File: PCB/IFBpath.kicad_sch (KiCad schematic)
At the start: 51 parts, among them J401 NC3FAH2, J402 Conn_01x03, J403 Conn_01x03, J404 Conn_01x03, J405 Conn_01x03, J406 NRJ6HF, J407 NRJ6HF, U401 THAT2162, U402 OPA1678, U403 OPA1622

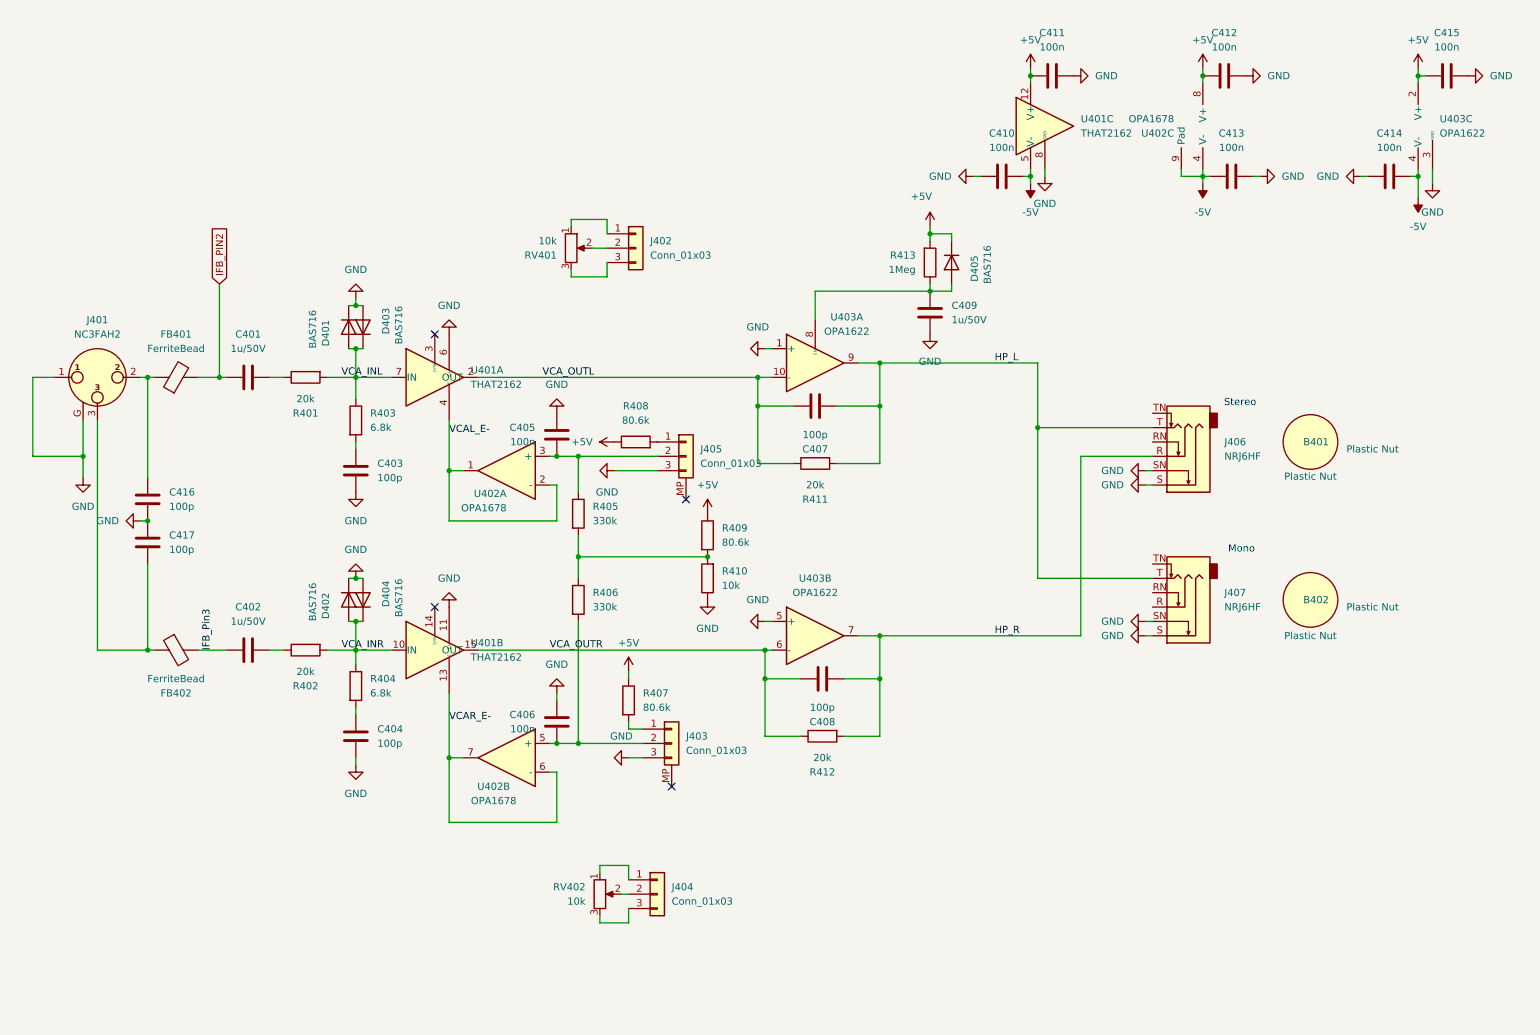
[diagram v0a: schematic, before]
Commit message: Tidying up
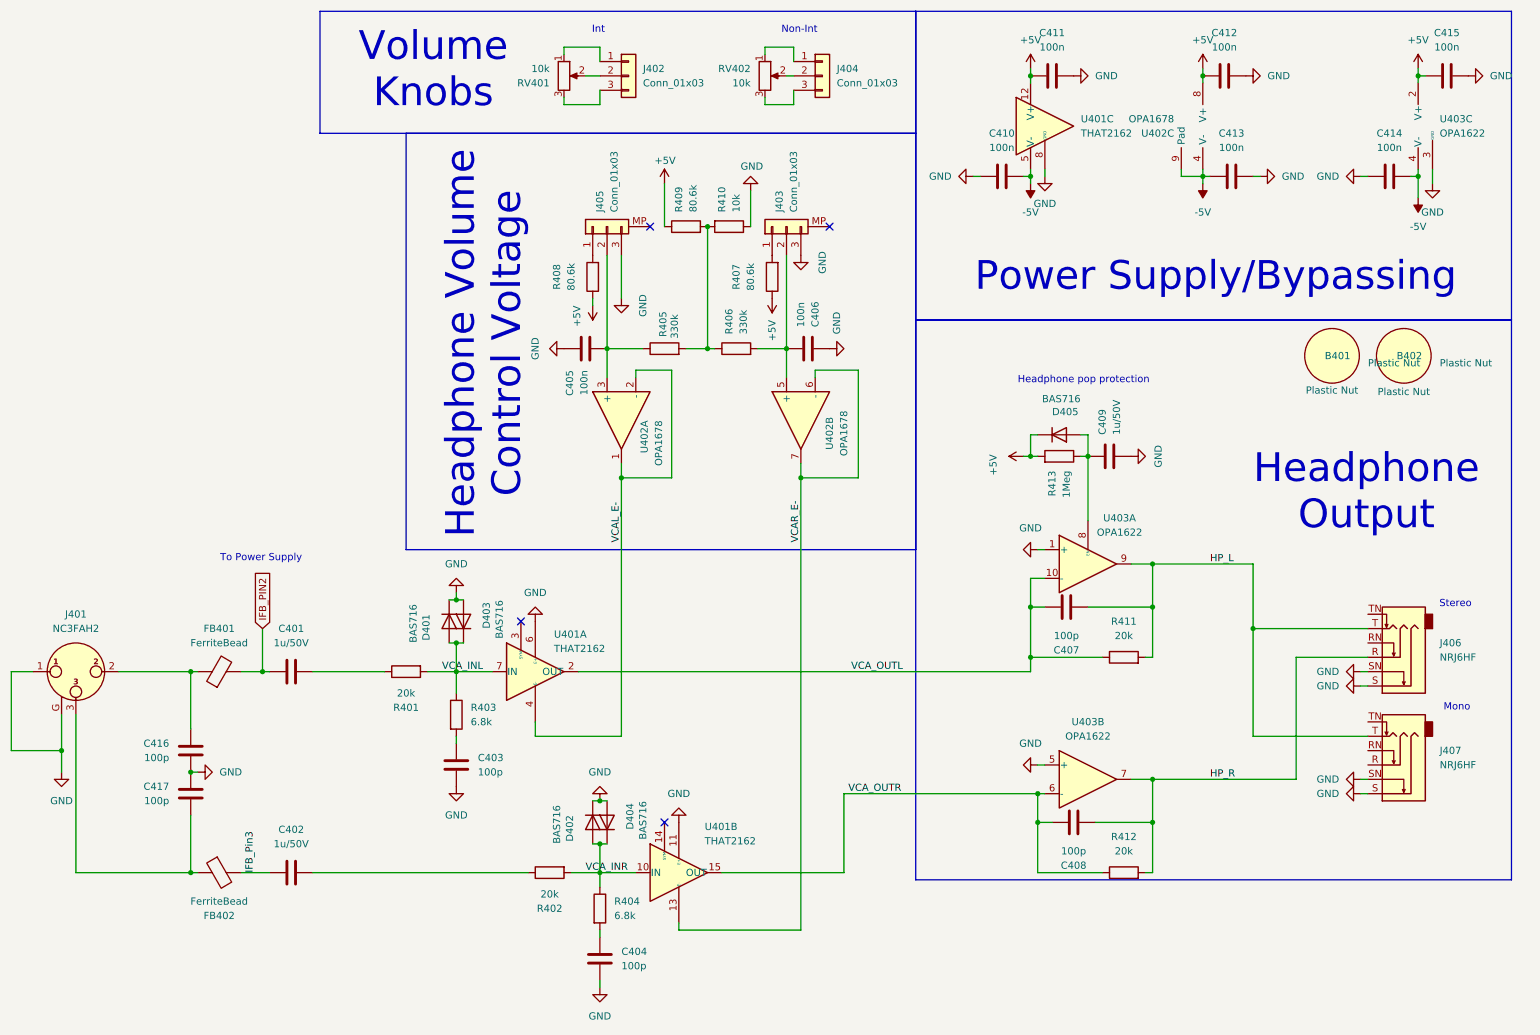
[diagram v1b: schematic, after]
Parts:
- U402: footprint STEVEannouncer:WSON-8-1EP_3x3mm_P0.5mm_EP1.2x2mm_ThermalVias -> Package_SON:WSON-8-1EP_3x3mm_P0.5mm_EP1.2x2mm_ThermalVias; Gearlabs Part Number (none) -> EXT-OPA1678
- U403: footprint STEVEannouncer:OPA1622 -> Package_SON:Texas_S-PVSON-N10
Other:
- note added: "Headphone Output"
- note added: "Headphone Volume Control Voltage"
- note added: "Headphone pop protection"
- note added: "Int"
- note added: "Non-Int"
- note added: "Power Supply/Bypassing"
- note added: "To Power Supply"
- note added: "Volume Knobs"
- moved on the sheet: B401, B402, C401, C402, C403, C404, C405, C406, C407, C408, C409, C416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
